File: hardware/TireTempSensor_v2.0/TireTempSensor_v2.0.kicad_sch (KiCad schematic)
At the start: 20 parts

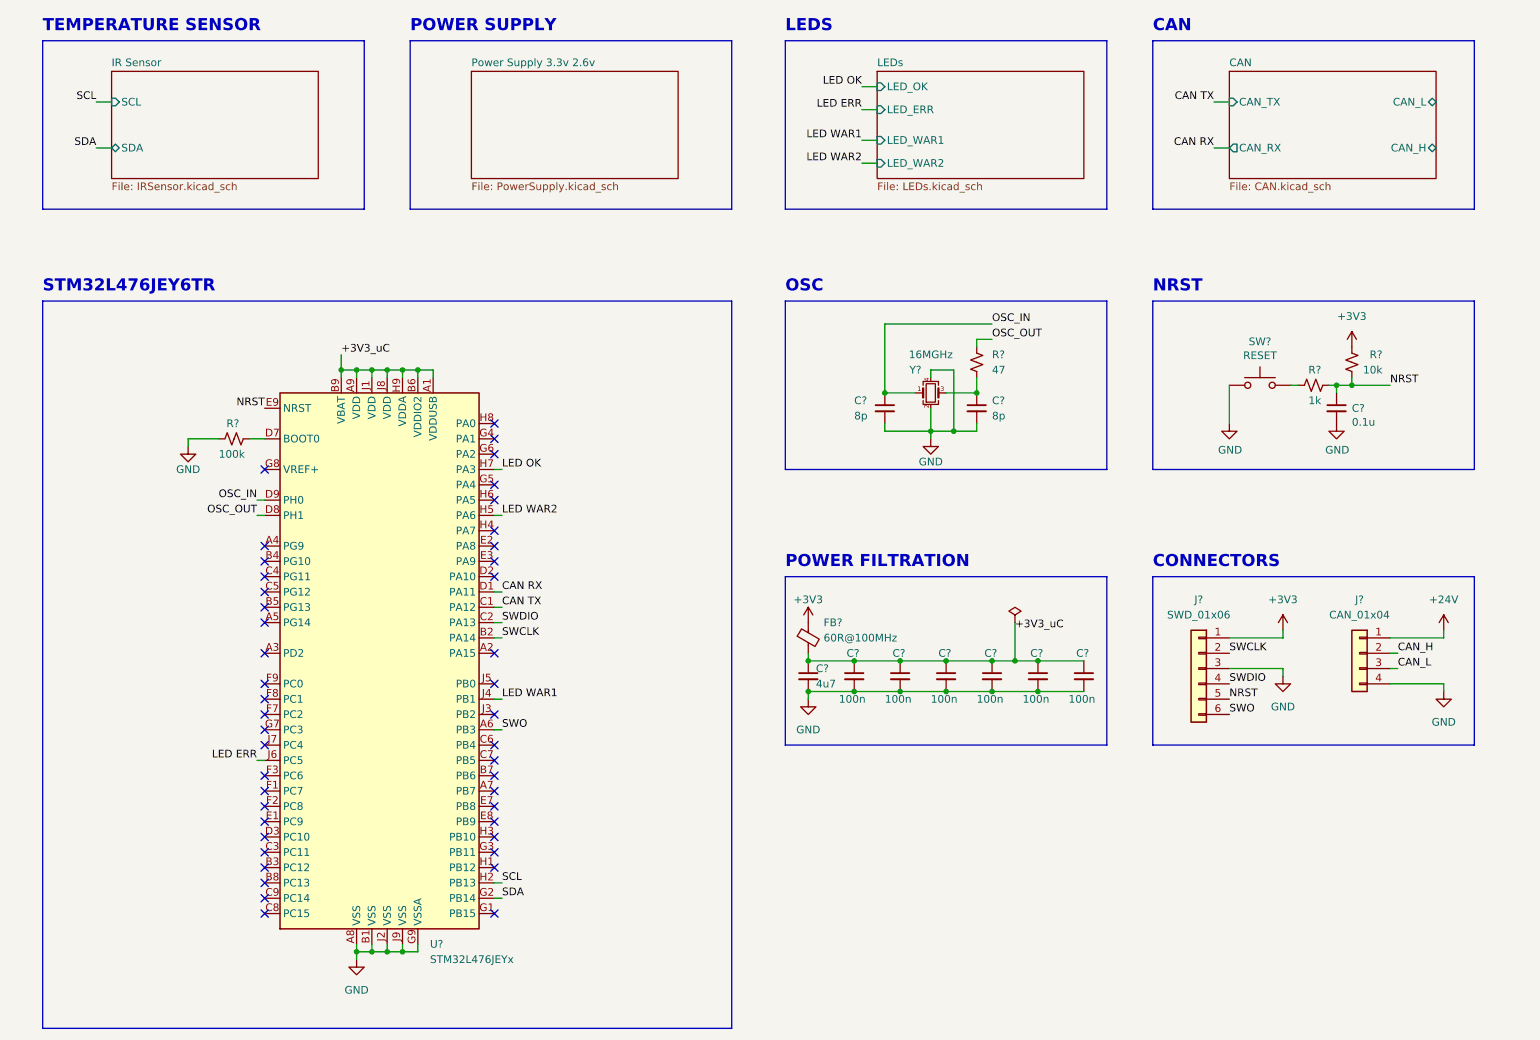
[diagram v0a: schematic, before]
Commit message: erc tests passed
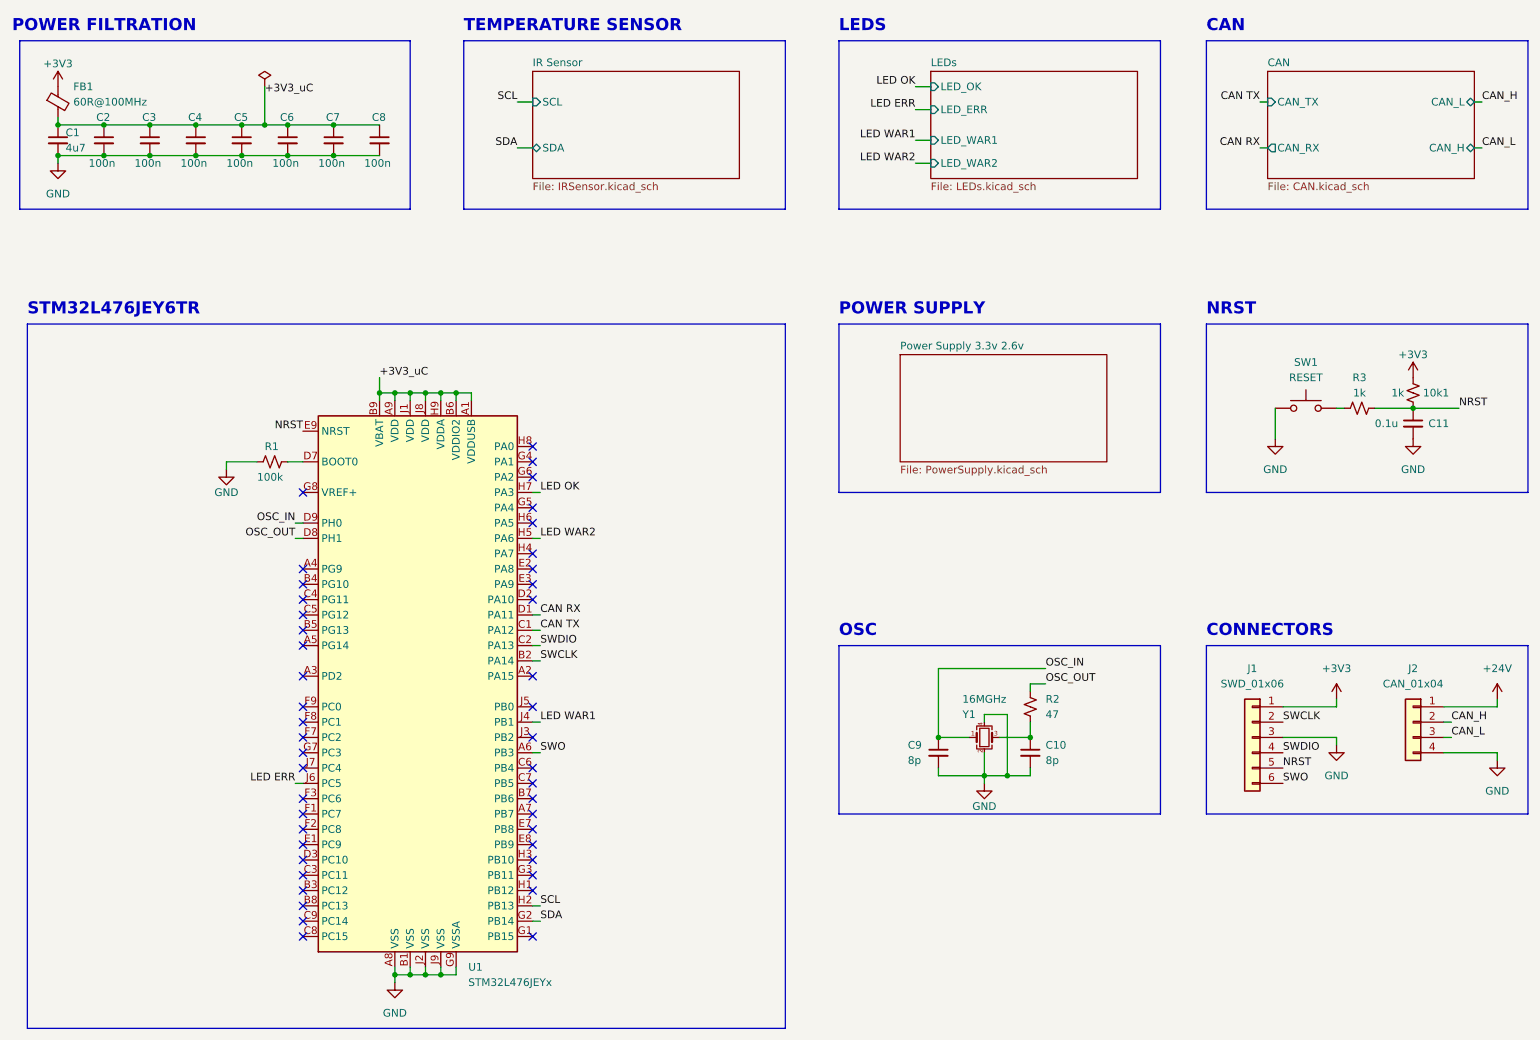
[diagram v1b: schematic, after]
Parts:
- removed C?: 0.1u, Capacitor_SMD:C_0603_1608Metric, symbol SB-Spoko-Bezpieczniki-rescue:C_Small-Device
- removed R?: 10k, Resistor_SMD:R_0603_1608Metric, symbol Device:R_Small_US
- removed R?: 1k, Resistor_SMD:R_0603_1608Metric, symbol Device:R_Small_US
- removed SW?: RESET, BUTTON:434781025816, symbol SB-Spoko-Bezpieczniki-rescue:SW_Push-Switch
- added 10k1, R3: 1k, symbol Device:R_Small_US
- added C11: 0.1u, symbol Device:C_Small
- added C8: 100n, Capacitor_SMD:C_0603_1608Metric, symbol Device:C_Small
- added SW1: RESET, symbol Switch:SW_MEC_5G
- gave numbers to parts that had none: 16
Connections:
- net +3V3: now also 10k1.2
- net +3V3_uC: now also C8.1
- net GND: now also C11.2, C8.2, SW1.1 (A), SW1.2 (A)
- net NRST: now also 10k1.1, C11.1, R3.2
- new net: R3.1, SW1.3 (B), SW1.4 (B)
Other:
- moved on the sheet: C1, C10, C2, C3, C4, C5, C6, C7, C9, FB1, J1, J2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
